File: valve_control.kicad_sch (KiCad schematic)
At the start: 1 part, among them U4 ULN2003V12

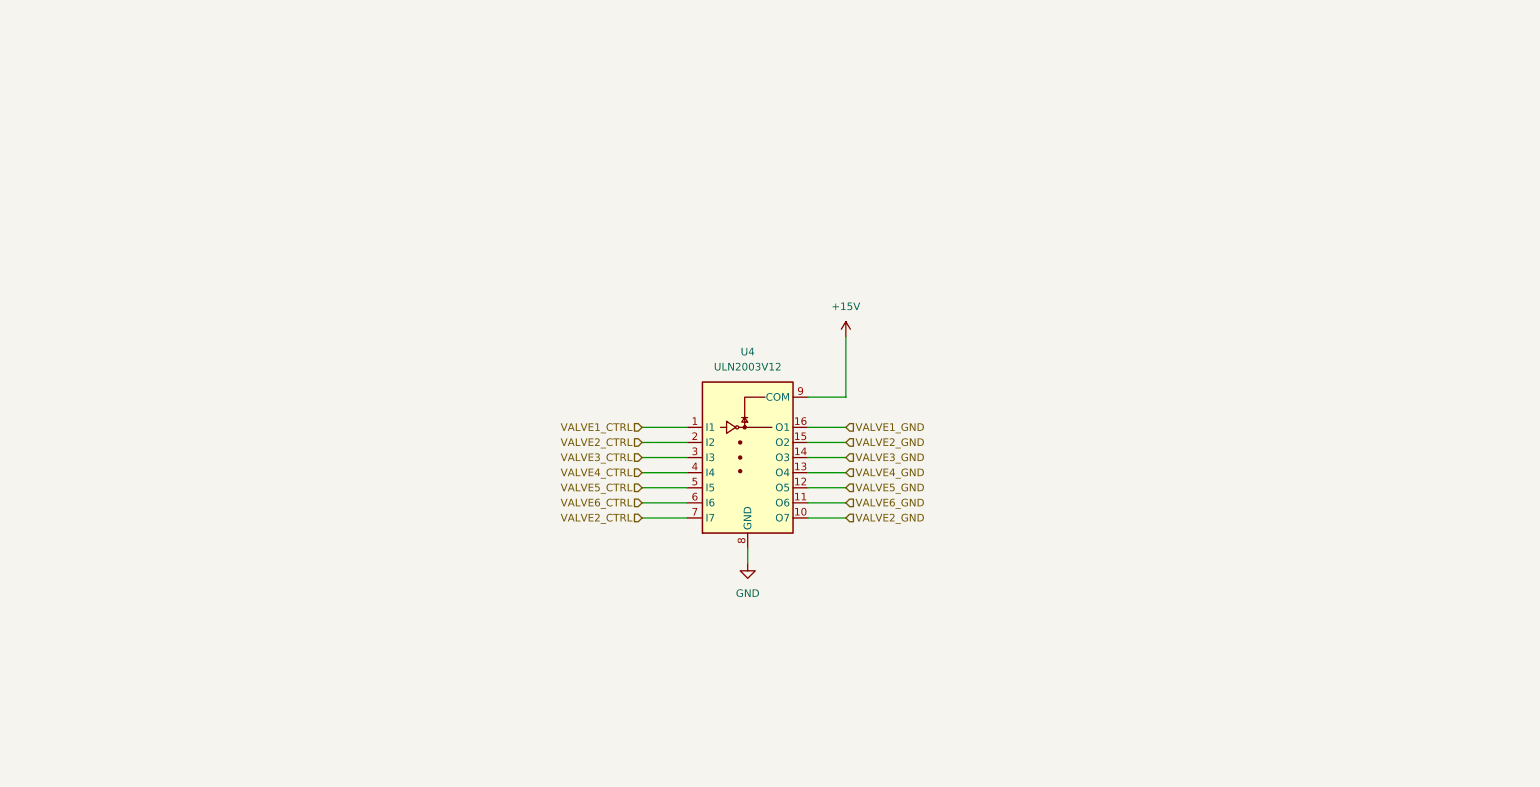
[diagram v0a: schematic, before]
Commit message: Finish first design
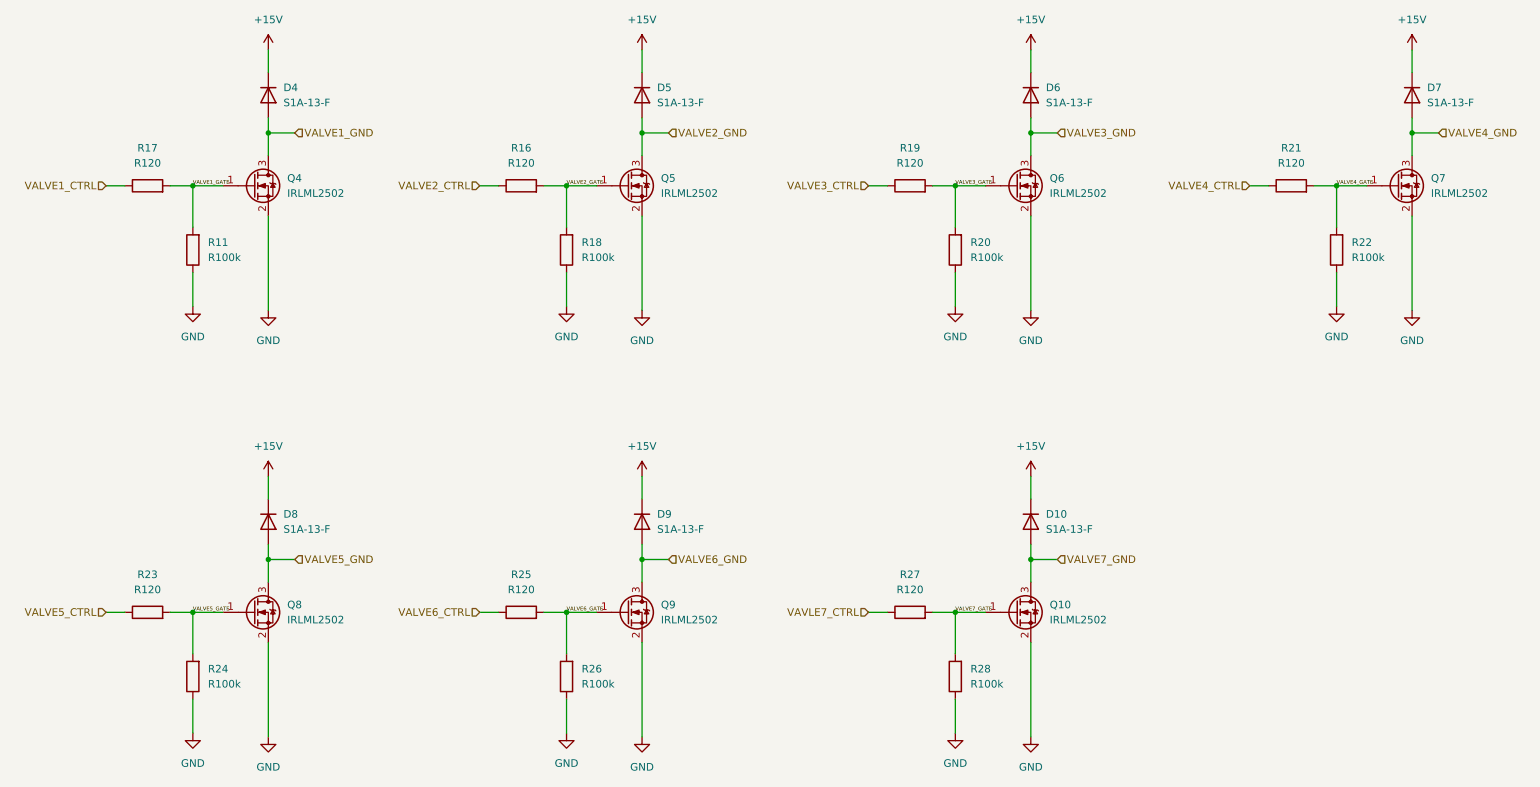
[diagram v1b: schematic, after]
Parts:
- removed U4: ULN2003V12, symbol Transistor_Array:ULN2003
- added D10, D4, D5, D6, D7, D8, D9: S1A-13-F, Diode_SMD:D_SMA, symbol Device:D
- added Q10, Q4, Q5, Q6, Q7, Q8, Q9: IRLML2502, Package_TO_SOT_SMD:SOT-23, symbol Device:Q_NMOS_GSD
- added R11, R18, R20, R22, R24, R26, R28: R100k, Resistor_SMD:R_0805_2012Metric, symbol Device:R
- added R16, R17, R19, R21, R23, R25, R27: R120, Resistor_SMD:R_0805_2012Metric, symbol Device:R
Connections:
- net +15V: now also D10.1 (K), D4.1 (K), D5.1 (K), D6.1 (K), D7.1 (K), D8.1 (K), D9.1 (K)
- net GND: now also Q10.2 (S), Q4.2 (S), Q5.2 (S), Q6.2 (S), Q7.2 (S), Q8.2 (S), Q9.2 (S), R11.1, R18.1, R20.1, R22.1, R24.1, R26.1, R28.1
- net VALVE1_CTRL: now also R17.1
- net VALVE1_GND: now also D4.2 (A), Q4.3 (D)
- net VALVE2_CTRL: now also R16.1
- net VALVE2_GND: now also D5.2 (A), Q5.3 (D)
- net VALVE3_CTRL: now also R19.1
- net VALVE3_GND: now also D6.2 (A), Q6.3 (D)
- net VALVE4_CTRL: now also R21.1
- net VALVE4_GND: now also D7.2 (A), Q7.3 (D)
- net VALVE5_CTRL: now also R23.1
- net VALVE5_GND: now also D8.2 (A), Q8.3 (D)
- net VALVE6_CTRL: now also R25.1
- net VALVE6_GND: now also D9.2 (A), Q9.3 (D)
- new net VALVE1_GATE: Q4.1 (G), R11.2, R17.2
- new net VALVE2_GATE: Q5.1 (G), R16.2, R18.2
- new net VALVE3_GATE: Q6.1 (G), R19.2, R20.2
- new net VALVE4_GATE: Q7.1 (G), R21.2, R22.2
- new net VALVE5_GATE: Q8.1 (G), R23.2, R24.2
- new net VALVE6_GATE: Q9.1 (G), R25.2, R26.2
- new net VALVE7_GATE: Q10.1 (G), R27.2, R28.2
- new net VALVE7_GND: D10.2 (A), Q10.3 (D)
- new net VAVLE7_CTRL: R27.1
